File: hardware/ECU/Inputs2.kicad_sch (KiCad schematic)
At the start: 9 parts, among them Q6 Q_DUAL_NMOS_S1G1D2S2G2D1, U11 LMV324LIDT

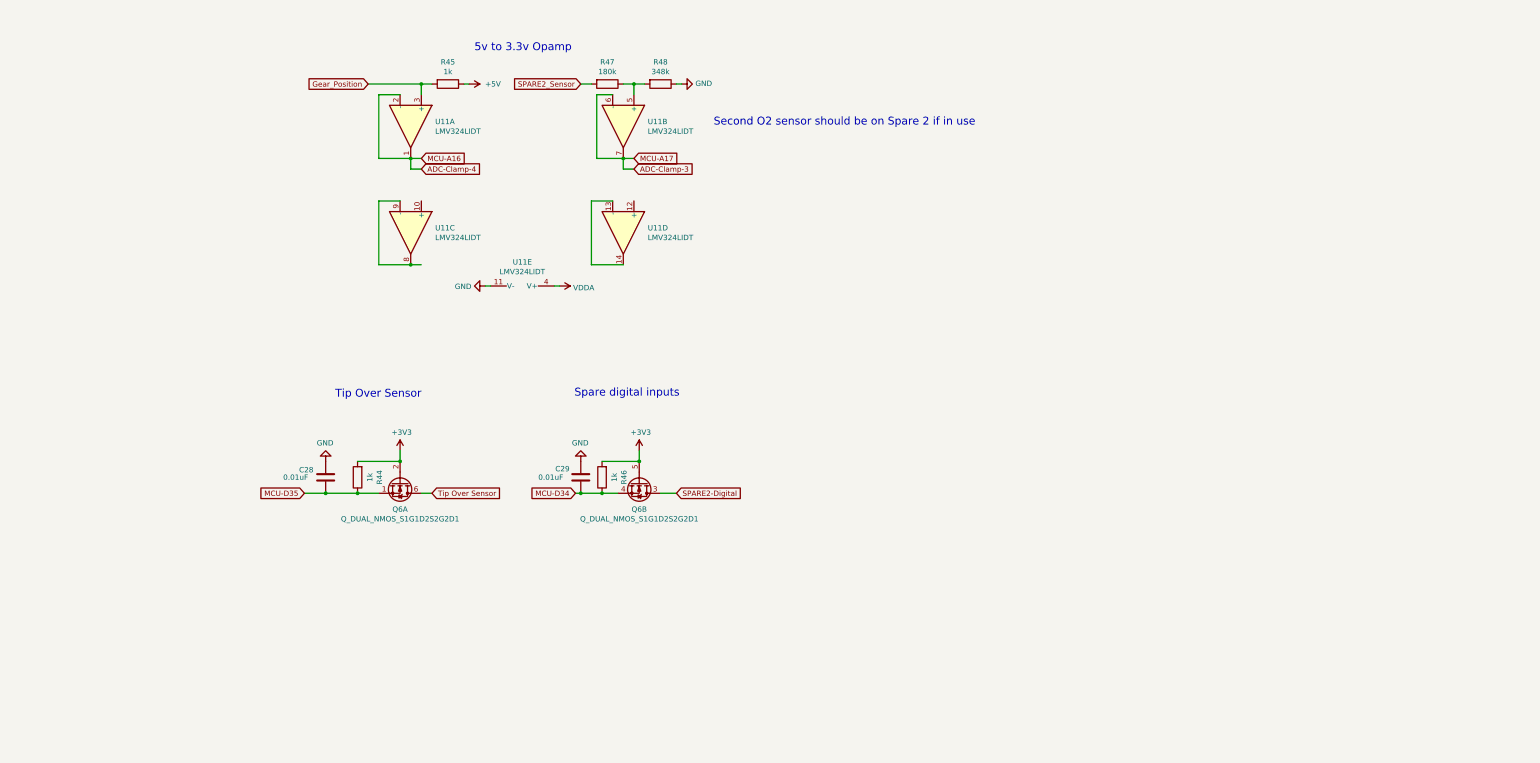
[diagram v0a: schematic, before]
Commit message: Update ECU-Hardware, Dokumente und Explosionszeichnungen
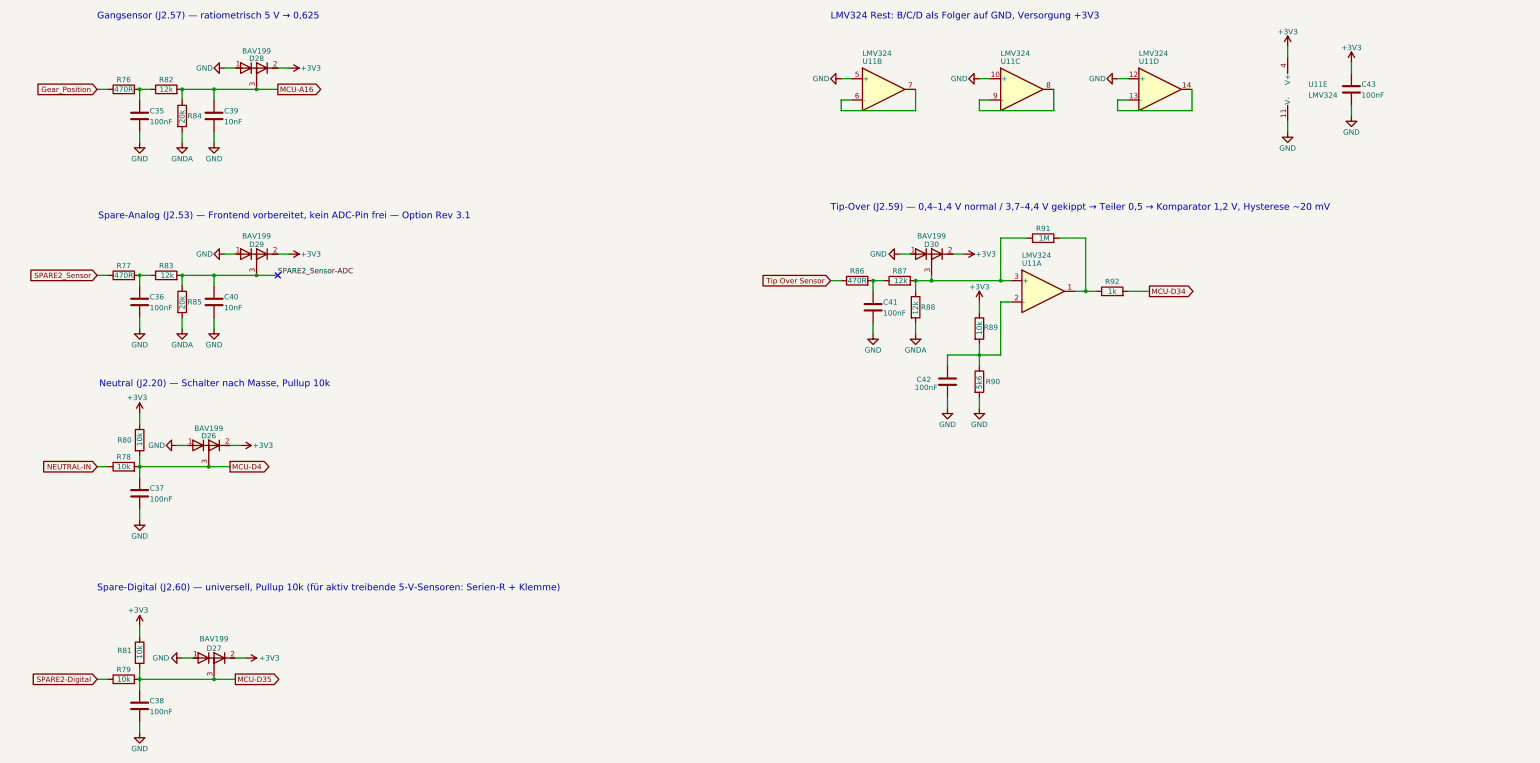
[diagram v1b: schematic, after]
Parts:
- removed C28, C29: 0.01uF, Capacitor_SMD:C_0805_2012Metric, symbol Device:C
- removed Q6: Q_DUAL_NMOS_S1G1D2S2G2D1, Package_TO_SOT_SMD:SOT-363_SC-70-6, symbol Device:Q_DUAL_NMOS_S1G1D2S2G2D1
- removed R44, R45, R46: 1k, Resistor_SMD:R_0805_2012Metric, symbol Device:R
- removed R47: 180k, Resistor_SMD:R_0805_2012Metric, symbol Device:R
- removed R48: 348k, Resistor_SMD:R_0805_2012Metric, symbol Device:R
- added C35, C36, C37, C38, C41, C42, C43: 100nF, Capacitor_SMD:C_0805_2012Metric, symbol Device:C
- added C39, C40: 10nF, Capacitor_SMD:C_0805_2012Metric, symbol Device:C
- added D26, D27, D28, D29, D30: BAV199, Package_TO_SOT_SMD:SOT-23, symbol Diode:BAV199
- added R76, R77, R86: 470R, Resistor_SMD:R_0805_2012Metric, symbol Device:R
- added R78, R79, R80, R81, R89: 10k, Resistor_SMD:R_0805_2012Metric, symbol Device:R
- added R82, R83, R87, R88: 12k, Resistor_SMD:R_0805_2012Metric, symbol Device:R
- added R84, R85: 20k, Resistor_SMD:R_0805_2012Metric, symbol Device:R
- added R90: 5k6, Resistor_SMD:R_0805_2012Metric, symbol Device:R
- added R91: 1M, Resistor_SMD:R_0805_2012Metric, symbol Device:R
- added R92: 1k, Resistor_SMD:R_0805_2012Metric, symbol Device:R
- U11: value LMV324LIDT -> LMV324; Digikey Part Number 497-13052-1-ND -> 296-9569-1-ND; Manufacturer_Name STMicroelectronics -> Texas Instruments; Manufacturer_Part_Number LMV324LIDT -> LMV324IDR; Supplier (none) -> DigiKey; URL https://www.digikey.com.au/product-detail/en/stmicroelectro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 -> (none)
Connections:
- net VDDA is gone; now on net +3V3: U11.4 (V+)
- net +3V3: now also C43.1, D26.2 (K2), D27.2 (K2), D28.2 (K2), D29.2 (K2), D30.2 (K2), R80.1, R81.1, R89.1
- net GND: now also U11.10 (+), U11.12 (+), U11.5 (+), C35.2, C36.2, C37.2, C38.2, C39.2, C40.2, C41.2, C42.2, C43.2, D26.1 (A1), D27.1 (A1), D28.1 (A1), D29.1 (A1), D30.1 (A1), R90.2
- net Gear_Position: now also R76.1; no longer U11.3 (+)
- net MCU-D34: now also R92.2
- net MCU-D35: now also C38.1, D27.3 (K1A2), R79.2, R81.2
- net SPARE2-Digital: now also R79.1
- net SPARE2_Sensor: now also R77.1
- net Tip Over Sensor: now also R86.1
- net ADC-Clamp-3: no longer names the net of U11.6 (-), U11.7
- net ADC-Clamp-4: no longer names the net of U11.2 (-)
- net ADC-Clamp-4: now also C42.1, R89.2, R90.1; no longer U11.1
- new net: D30.3 (K1A2), R87.2, R88.1, R91.1, U11.3 (+)
- new net: C41.1, R86.2, R87.1
- new net: R91.2, R92.1, U11.1
- new net: C36.1, R77.2, R83.1
- new net: C35.1, R76.2, R82.1
- new net GNDA: R84.2, R85.2, R88.2
- new net MCU-A16: C39.1, D28.3 (K1A2), R82.2, R84.1
- new net MCU-D4: C37.1, D26.3 (K1A2), R78.2, R80.2
- new net NEUTRAL-IN: R78.1
- new net SPARE2_Sensor-ADC: C40.1, D29.3 (K1A2), R83.2, R85.1
- no-connect marks 0 -> 1
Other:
- note added: "Gangsensor (J2.57) — ratiometrisch 5 V → 0,625"
- note added: "LMV324 Rest: B/C/D als Folger auf GND, Versorgung +3V3"
- note added: "Neutral (J2.20) — Schalter nach Masse, Pullup 10k"
- note added: "Spare-Analog (J2.53) — Frontend vorbereitet, kein ADC-Pin frei — Option Rev 3.1"
- note added: "Spare-Digital (J2.60) — universell, Pullup 10k (für aktiv treibende 5-V-Sensoren: Serien-R + Klemme)"
- note added: "Tip-Over (J2.59) — 0,4–1,4 V normal / 3,7–4,4 V gekippt → Teiler 0,5 → Komparator 1,2 V, Hysterese ~20 mV"
- note removed: "5v to 3.3v Opamp"
- note removed: "Second O2 sensor should be on Spare 2 if in use"
- note removed: "Spare digital inputs"
- note removed: "Tip Over Sensor"
- title: (none) -> Inputs 2
